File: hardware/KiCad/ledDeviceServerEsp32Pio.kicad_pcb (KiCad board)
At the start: 2 copper layers, 81 x 76 mm, 12 parts, among them U1 ESP32-DevKitC, U2 LLC_4CH

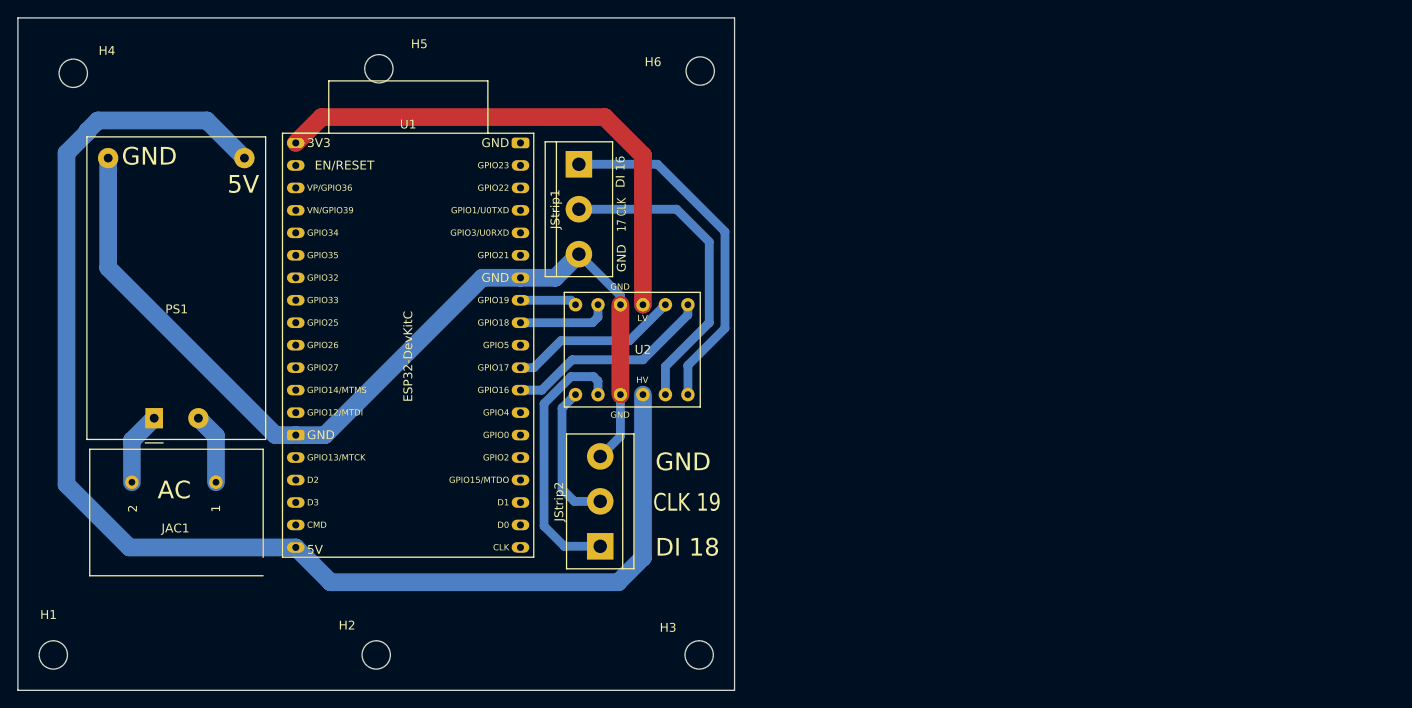
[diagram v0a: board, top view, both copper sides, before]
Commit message: adding long-pcb
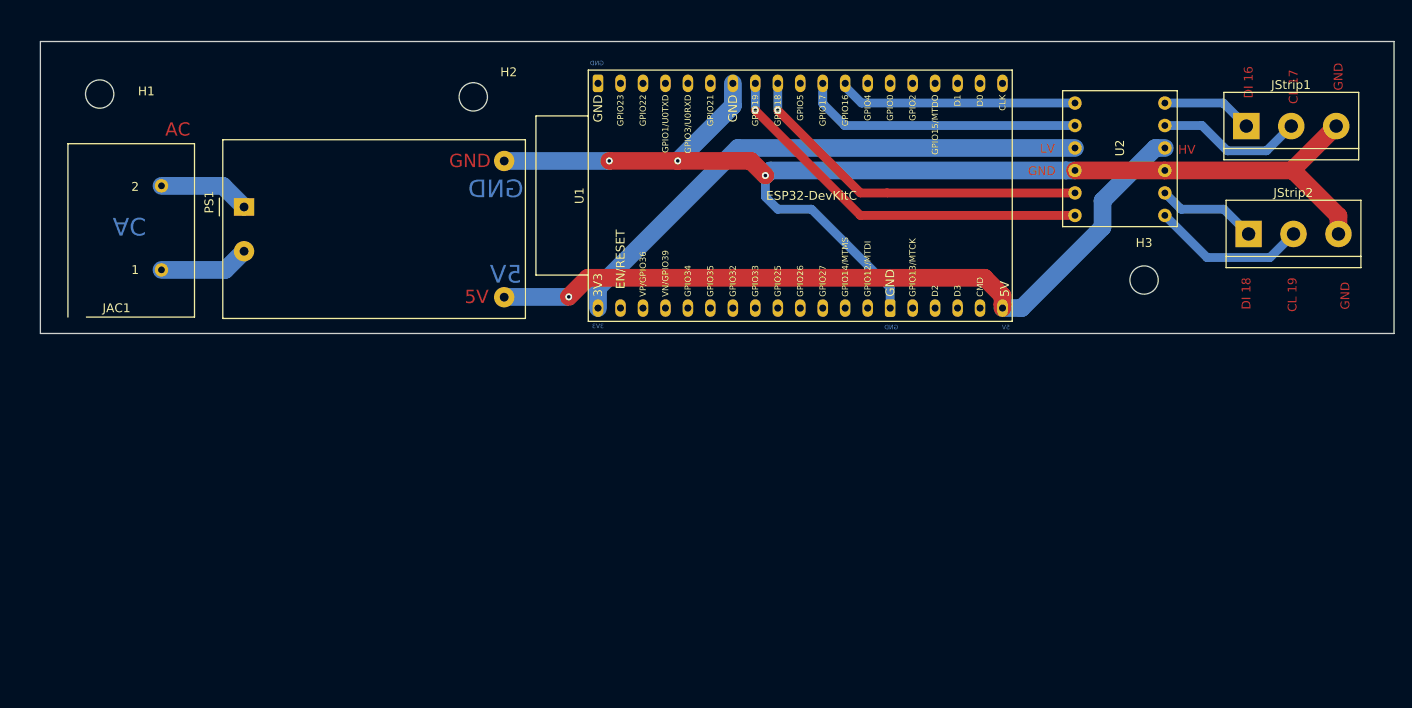
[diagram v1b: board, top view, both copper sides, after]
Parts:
- removed H4, H5, H6: MountingHole, MountingHole:MountingHole_3.2mm_M3
- moved JStrip2 81.3 mm to (149.1, 34.4), turned to 0 degrees
- moved JStrip1 75.6 mm to (148.8, 22.2), turned to 0 degrees
- moved H3 65.8 mm to (137.3, 39.6)
- moved U2 64.7 mm to (141.0, 18.2), turned to 270 degrees
- moved H2 64.0 mm to (61.5, 18.9)
- moved H1 63.6 mm to (19.2, 18.6)
- moved U1 38.9 mm to (75.6, 42.8), turned to 90 degrees
- moved PS1 25.9 mm to (35.6, 31.4), turned to 0 degrees
- moved JAC1 19.1 mm to (28.3, 43.8), turned to 180 degrees
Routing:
- net Net-(PS1-Pad4): track 150.2 -> 87.1 mm, vias 0 -> 1
- net Net-(U1-Pad31): track 6.43 -> 44.1 mm, vias 0 -> 1
- net GND: track 107.7 -> 140.9 mm, vias 0 -> 3
- net Net-(U1-Pad30): track 10.4 -> 40.5 mm, vias 0 -> 1
- net /DATA1: track 39.8 -> 10.3 mm
- net /CLOCK1: track 35.6 -> 16.6 mm
- net /DATA2: track 30.2 -> 11.4 mm
- net Net-(U1-Pad28): track 19.3 -> 31.8 mm
- net Net-(U1-Pad1): track 59.1 -> 62.7 mm
- net Net-(U1-Pad27): track 23.6 -> 27.1 mm
- net Net-(JAC1-Pad1): track 8.06 -> 10.2 mm
- net Net-(JAC1-Pad2): track 8.28 -> 10.3 mm
- net /CLOCK2: track 16.2 -> 17.6 mm
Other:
- board size 81 x 76 mm -> 153 x 33 mm
- board text added: "3V3"
- board text added: "CL 17"
- board text added: "CL 19"
- board text removed: "17 CLK"
- board text removed: "CLK 19"
